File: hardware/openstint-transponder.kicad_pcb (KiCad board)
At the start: 4 copper layers, 18.5 x 16 mm, 33 parts, among them J1 V+, J2 V-, Q1 AO3401A, U1 STM32C011F4Ux, U3 UCC27517DBV, U4 TLV760xx, Y1 20 MHz

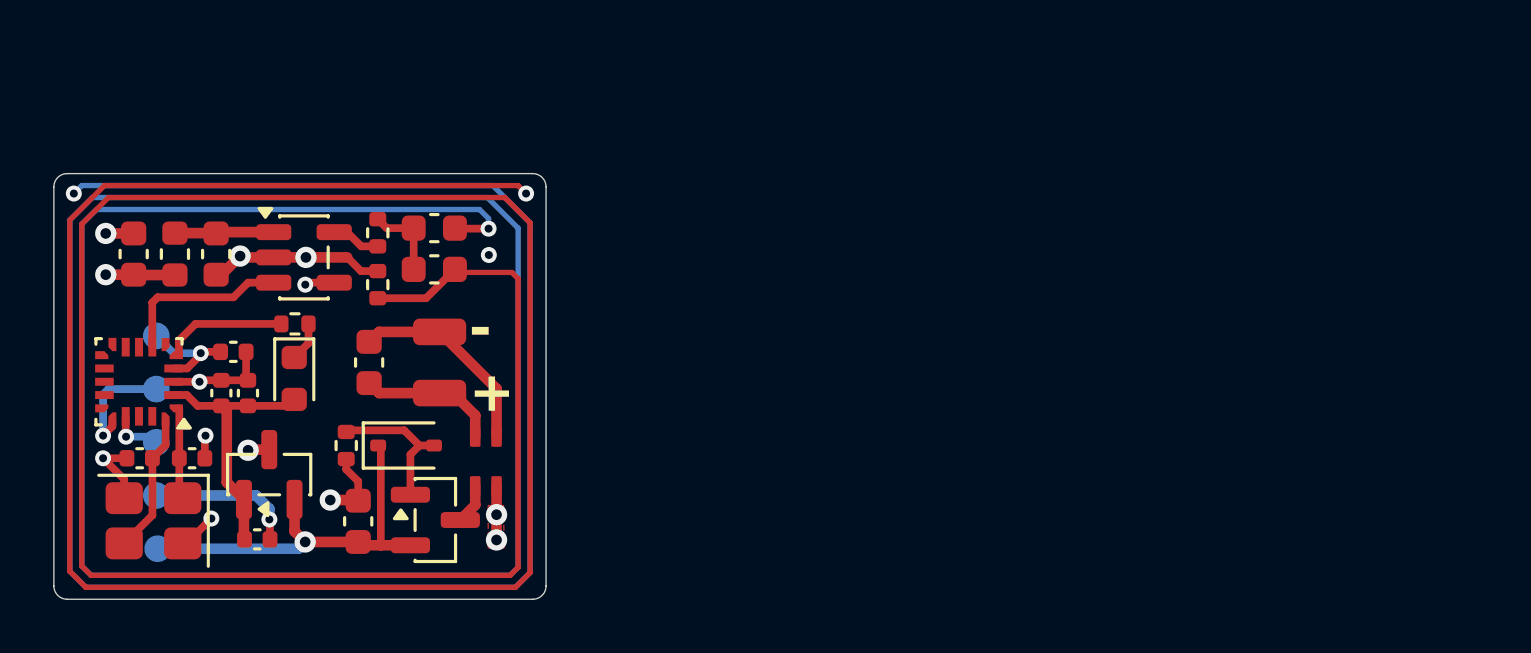
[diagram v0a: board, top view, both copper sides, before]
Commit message: v2 transponder
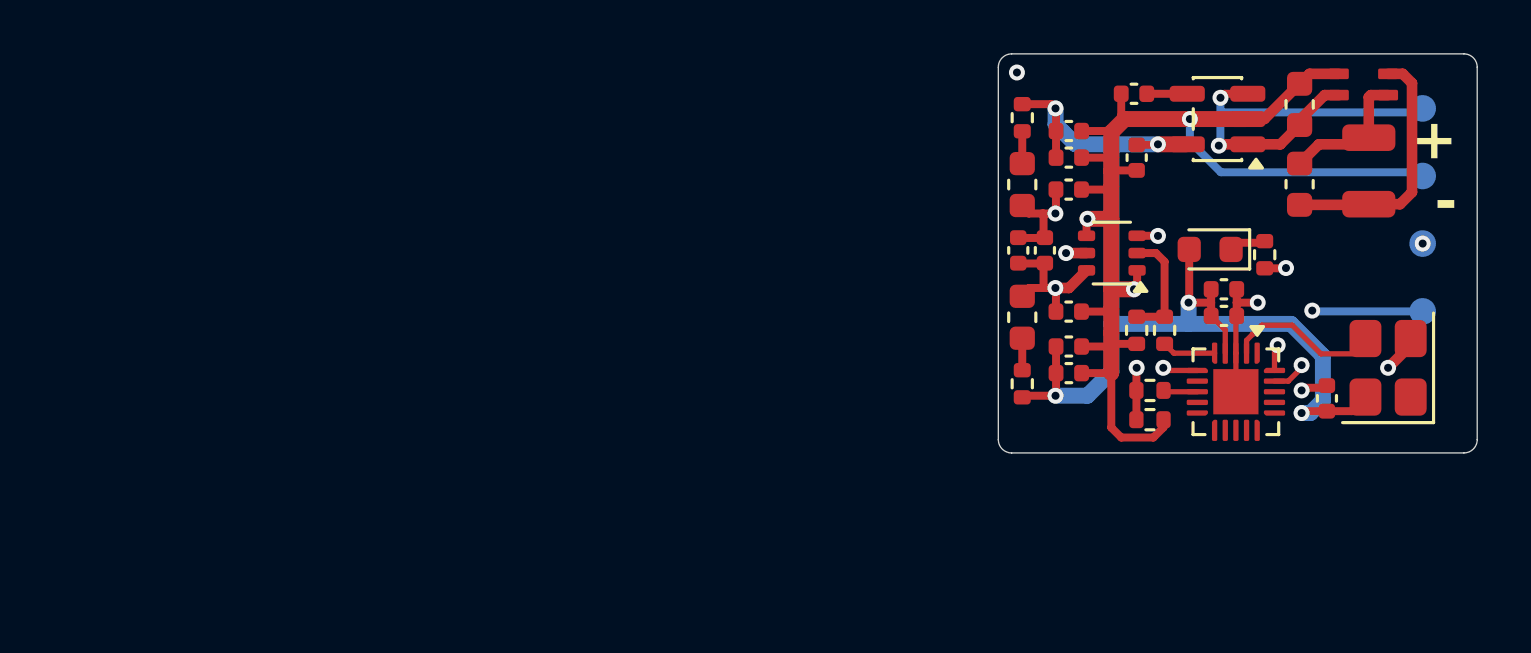
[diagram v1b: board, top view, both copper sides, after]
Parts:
- removed D2: 9.1V, Diode_SMD:D_SOD-323
- removed L1: 68n, Inductor_SMD:L_0603_1608Metric
- removed TP5: TestPoint, TestPoint:TestPoint_Pad_D1.0mm
- removed U4: TLV760xx, Package_TO_SOT_SMD:SOT-23
- removed Y1: 20 MHz, Crystal:Crystal_SMD_3225-4Pin_3.2x2.5mm
- added C13: 22p, Capacitor_SMD:C_0402_1005Metric, F.Cu at (132.6, 104.7)
- added C14: 22p, Capacitor_SMD:C_0402_1005Metric, F.Cu at (132.6, 100.1)
- added C15: 10u, Capacitor_SMD:C_0402_1005Metric, F.Cu at (132.7, 106.0)
- added L2: 3.3u, Inductor_SMD:L_0603_1608Metric, F.Cu at (130.9, 104.9)
- added L3: 3.3u, Inductor_SMD:L_0603_1608Metric, F.Cu at (130.9, 99.9)
- added R4: 22, Resistor_SMD:R_0402_1005Metric, F.Cu at (130.9, 97.4)
- added R6: 100k, Resistor_SMD:R_0402_1005Metric, F.Cu at (135.2, 105.4)
- added R7: 100k, Resistor_SMD:R_0402_1005Metric, F.Cu at (135.7, 108.8)
- added U2: 10 MHz, Crystal:Crystal_SMD_3225-4Pin_3.2x2.5mm, F.Cu at (144.7, 106.8)
- C1: value 4.7u/16V -> 10u; footprint Capacitor_SMD:C_0603_1608Metric -> Capacitor_SMD:C_0402_1005Metric
- C10: value 4.7u/16V -> 100n; footprint Capacitor_SMD:C_0603_1608Metric -> Capacitor_SMD:C_0402_1005Metric
- C11: value 680p -> 1n; footprint Capacitor_SMD:C_0603_1608Metric -> Capacitor_SMD:C_0402_1005Metric
- C4: value 20p -> 100n
- C5: value 20p -> 10n
- C6: value 470p -> 1n; footprint Capacitor_SMD:C_0603_1608Metric -> Capacitor_SMD:C_0402_1005Metric
- Q1: value AO3401A -> PMGD280UN; footprint Package_TO_SOT_SMD:SOT-23 -> Package_TO_SOT_SMD:SOT-363_SC-70-6
- R1: value 220 -> 22
- R3: value 0 -> 22
- U1: value STM32C011F4Ux -> ATtiny1616-M; footprint Package_DFN_QFN:ST_UFQFPN-20_3x3mm_P0.5mm -> Package_DFN_QFN:VQFN-20-1EP_3x3mm_P0.4mm_EP1.7x1.7mm
- U3: value UCC27517DBV -> SPX3819M5-L-3-3
- moved TP3 50.3 mm to (145.9, 97.0), turned to 90 degrees
- moved TP4 49.1 mm to (145.9, 99.6), turned to 90 degrees
- moved TP1 47.7 mm to (145.9, 102.1), turned to 90 degrees
- moved TP2 47.7 mm to (145.9, 104.7), turned to 180 degrees
- moved C4 44.7 mm to (142.3, 108.0), turned to -90 degrees
- moved U1 41.2 mm to (138.9, 107.7), turned to -90 degrees
- moved C7 38.7 mm to (141.3, 96.9)
- moved C5 38.0 mm to (135.1, 96.5)
- moved C3 37.8 mm to (138.5, 104.8), turned to 180 degrees
- moved C12 36.9 mm to (138.5, 103.8), turned to 0 degrees
- moved R5 36.5 mm to (140.0, 102.5), turned to 90 degrees
- moved J1 36.2 mm to (143.9, 98.2)
- moved C9 36.0 mm to (135.2, 98.9), turned to -90 degrees
- moved FL1 35.9 mm to (143.7, 96.2), turned to 180 degrees
- moved C8 35.6 mm to (141.3, 99.9), turned to -90 degrees
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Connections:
- C1 pad 1: /V_PUSHPULL -> +3.3V
- C10 pad 1: VDDA -> GND
- C10 pad 2: GND -> +3.3V
- C11 pad 1: Net-(C11-Pad1) -> /A+
- C11 pad 2: /ANTENNA_LOOP -> /A-
- C2 pad 1: /~{RST} -> GND
- C2 pad 2: GND -> +3.3V
- C4 pad 2: Net-(U1-PC14) -> +3.3V
- C5 pad 1: GND -> Net-(U3-BP)
- C5 pad 2: Net-(U1-PC15) -> GND
- C6 pad 1: /ANTENNA_LOOP -> /A+
- C6 pad 2: Net-(C11-Pad1) -> /A-
- FL1 pad 1: /VIN- -> /VIN+
- FL1 pad 2: /VIN+ -> /VIN-
- FL1 pad 3: /VFILT+ -> GND
- FL1 pad 4: GND -> VDDA
- Q1 pad 1: /revpol_gate -> GND
- Q1 pad 2: VDDA -> /GANT+
- Q1 pad 3: /VFILT+ -> /A-
- R1 pad 1: GND -> /ANT+
- R1 pad 2: /revpol_gate -> /GANT+
- R2 pad 1: Net-(U3-OUT) -> /GANT-
- R2 pad 2: Net-(C11-Pad1) -> /ANT-
- R3 pad 1: GND -> Net-(L2-Pad1)
- R3 pad 2: /ANTENNA_LOOP -> +3.3V
- TP1 pad 1: /~{RST} -> /UDPI
- TP2 pad 1: /SWDIO -> /UART0TXD
- U1 pad 1: Net-(U1-PC15) -> unconnected-(U1-PA2-Pad1)
- U1 pad 16: /SWDIO -> unconnected-(U1-PC1-Pad16)
- U1 pad 17: /SWCLK -> unconnected-(U1-PC2-Pad17)
- U1 pad 19: unconnected-(U1-PB7-Pad19) -> /UDPI
- U1 pad 2: +3.3V -> /EXTCLK
- U1 pad 20: Net-(U1-PC14) -> /UART0TXD
- U1 pad 4: /~{RST} -> +3.3V
- U1 pad 5: /~{BLINKY} -> /ANT+
- U1 pad 6: unconnected-(U1-PA1-Pad6) -> /~{BLINKY}
- U1 pad 7: /ANT_IN -> unconnected-(U1-PA6-Pad7)
- U1 pad 8: unconnected-(U1-PA3-Pad8) -> /ANT-
- U3 pad 1: /V_PUSHPULL -> VDDA
- U3 pad 3: /ANT_IN -> VDDA
- U3 pad 4: GND -> Net-(U3-BP)
- U3 pad 5: Net-(U3-OUT) -> +3.3V
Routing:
- net GND: track 44.2 -> 78.9 mm, vias 13 -> 6
- net +3.3V: track 10.2 -> 43.8 mm, vias 0 -> 5
- net VDDA: track 32.6 -> 16.2 mm
- net /A-: track 0.00 -> 9.25 mm, vias 0 -> 3
- net /GANT-: track 0.00 -> 9.20 mm, vias 0 -> 2
- net /UDPI: track 0.00 -> 7.81 mm, vias 0 -> 2
- net /UART0TXD: track 0.00 -> 7.00 mm, vias 0 -> 2
- net /ANT_IN: track 6.55 -> 0.00 mm
- net /A+: track 0.00 -> 5.69 mm, vias 0 -> 1
- net /EXTCLK: track 0.00 -> 5.57 mm
- net /revpol_gate: track 5.55 -> 0.00 mm
- net /~{BLINKY}: track 4.67 -> 10.0 mm, vias 0 -> 2
- net Net-(U1-PC14): track 5.24 -> 0.00 mm
- net /ANTENNA_LOOP: track 4.62 -> 0.00 mm, vias 4 -> 0
- net /SWDIO: track 4.33 -> 0.00 mm, vias 1 -> 0
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- removed copper zone on F.Cu, net GND
- removed copper zone on In1.Cu, net GND
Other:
- board size 18.5 x 16 mm -> 18 x 15 mm
- board text added: "TxD"
- board text added: "UDPI"
- board text added: "VDD"
- board text removed: "CLK"
- board text removed: "DIO"
- board text removed: "RST"
- board text removed: "VCC"
